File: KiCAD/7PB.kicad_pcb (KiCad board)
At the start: 2 copper layers, 124.7 x 18 mm, 44 parts, among them J1 Connector, J2 Connector, Q1 BC547, Q2 BC547, Q3 BC547, Q4 BC547, Q5 BC547, Q6 BC547, Q7 BC547

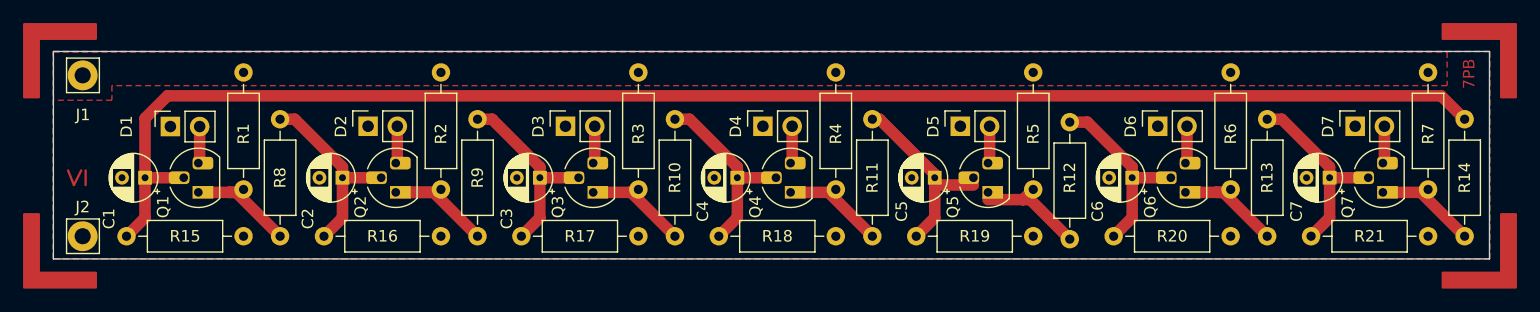
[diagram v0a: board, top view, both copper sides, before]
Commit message: Update
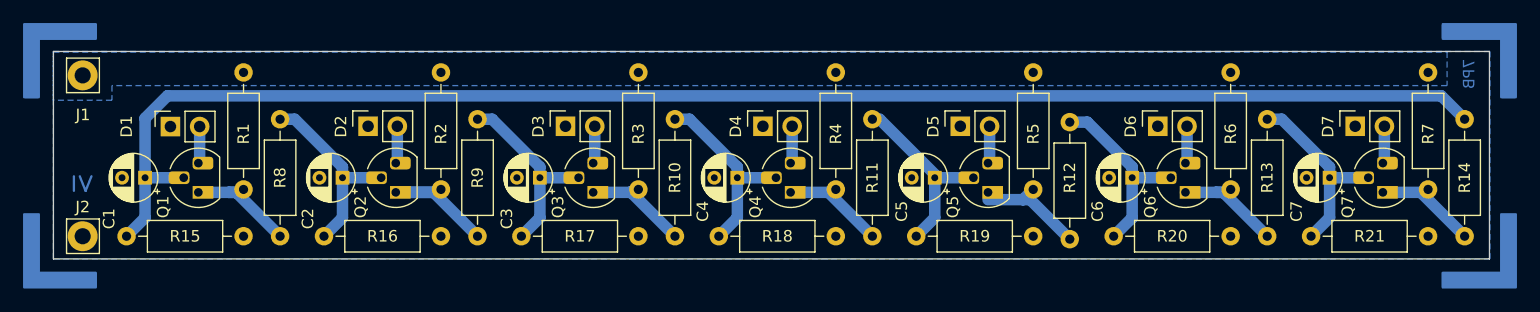
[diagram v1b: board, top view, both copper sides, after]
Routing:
- added copper zone on B.Cu, net +9V
- removed copper zone on F.Cu, net +9V
- removed copper zone on F.Cu, net GND
